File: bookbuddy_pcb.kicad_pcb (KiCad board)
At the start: 2 copper layers, 70 x 15 mm, 49 parts, among them IC1 APX810S-31SA-7, IC2 LM66200DRLR, J1 SM04B-SRSS-TB, J2 10164359-00011LF, J3 Battery Connector, Q1 DMG2305UX-13, SW1 SW_Push, SW2 SW_Push, SW3 SLW-66527511-SMT-TR, U1 ESP32-C3-MINI-1, U2 MLX90395KDC-BBA-101-RE, U3 MIC5504-3.3YM5-TR, U4 MCP73832, Y1 32.768kHz

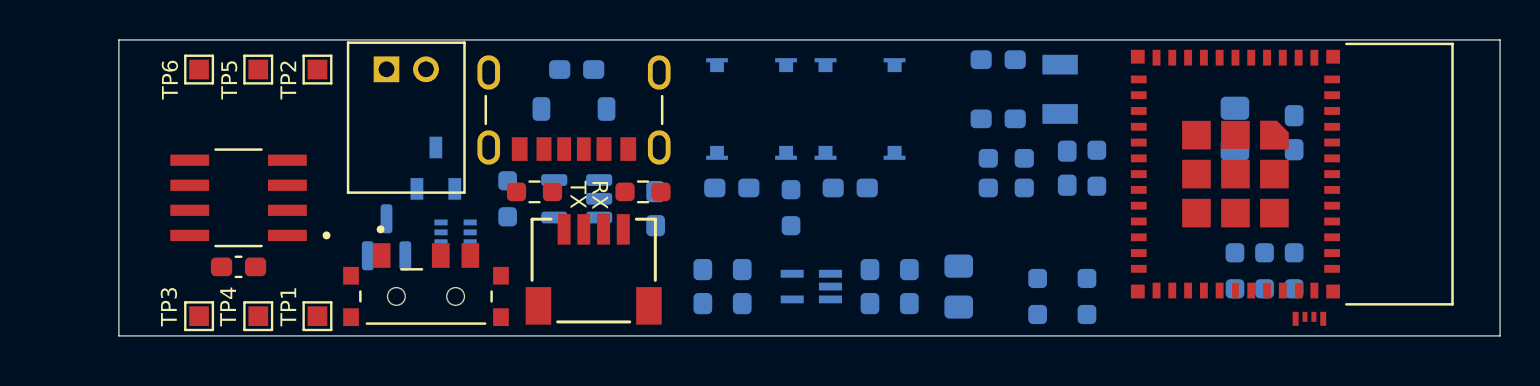
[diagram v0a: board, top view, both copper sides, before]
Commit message: Added fuse
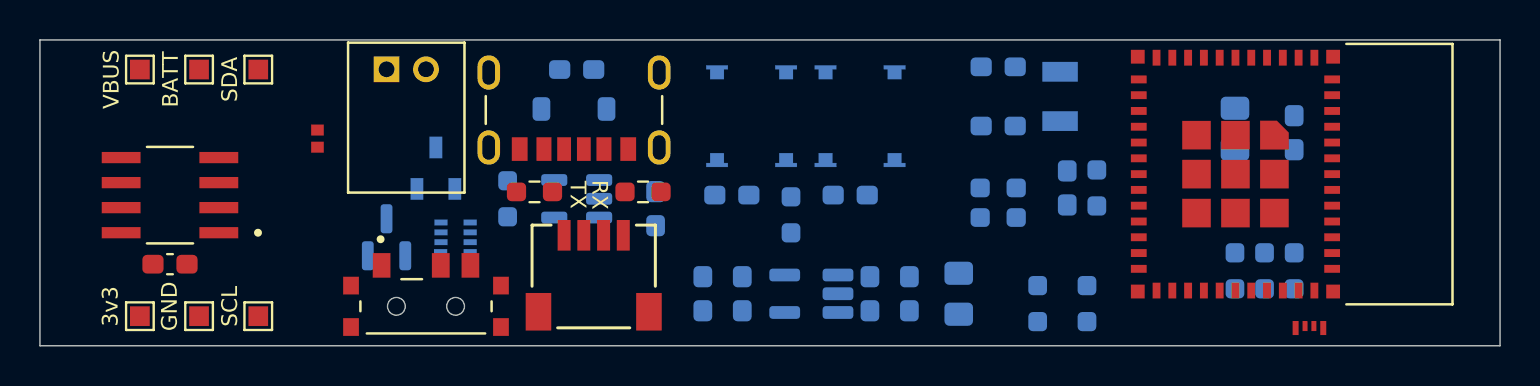
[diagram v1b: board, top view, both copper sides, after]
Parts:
- added F1: Fuse_Small, bookbuddy:FUSC0402X49N, F.Cu at (109.5, 90.5)
- U3: footprint bookbuddy:SOT65P210X110-5N -> Package_TO_SOT_SMD:SOT-23-5_HandSoldering
- moved C8 3.48 mm to (102.0, 96.9)
- moved U2 3.48 mm to (102.0, 93.4)
- moved 3v3 3.00 mm to (100.5, 99.5)
- moved BATT 3.00 mm to (103.5, 87.0)
- moved GND 3.00 mm to (103.5, 99.5)
- moved SCL 3.00 mm to (106.5, 99.5)
- moved SDA 3.00 mm to (106.5, 87.0)
- moved VBUS 3.00 mm to (100.5, 87.0)
- moved R11 1.56 mm to (144.0, 93.0)
- moved R12 1.56 mm to (144.0, 94.5)
- moved C13 1.00 mm to (147.5, 93.0)
- moved R2 1.00 mm to (149.0, 93.0)
- moved SW3 0.50 mm to (115.0, 99.0)
- moved LED1 0.47 mm to (159.8, 100.4)
- moved C1 0.36 mm to (144.0, 86.9)
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- renumbered TP3 to 3v3, TP5 to BATT, TP4 to GND, TP1 to SCL, TP2 to SDA, TP6 to VBUS
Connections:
- J3 pad 1: +BATT -> Net-(J3-Pin_1)
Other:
- board size 70 x 15 mm -> 74 x 15.5 mm
- board text added: "15.5mm"
- board text removed: "15mm"
